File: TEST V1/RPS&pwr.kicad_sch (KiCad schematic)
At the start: 42 parts, among them J10 Conn_01x01_Pin, J12 Conn_01x01_Pin, J7 Conn_01x01_Pin, J8 Conn_01x01_Pin, J9 Conn_01x01_Pin, Q2 PMOS, U11 TVS1800DRV, U12 TPS54202DDC, U13 MCP4725A2T-ECH, U6 LM2596T-5

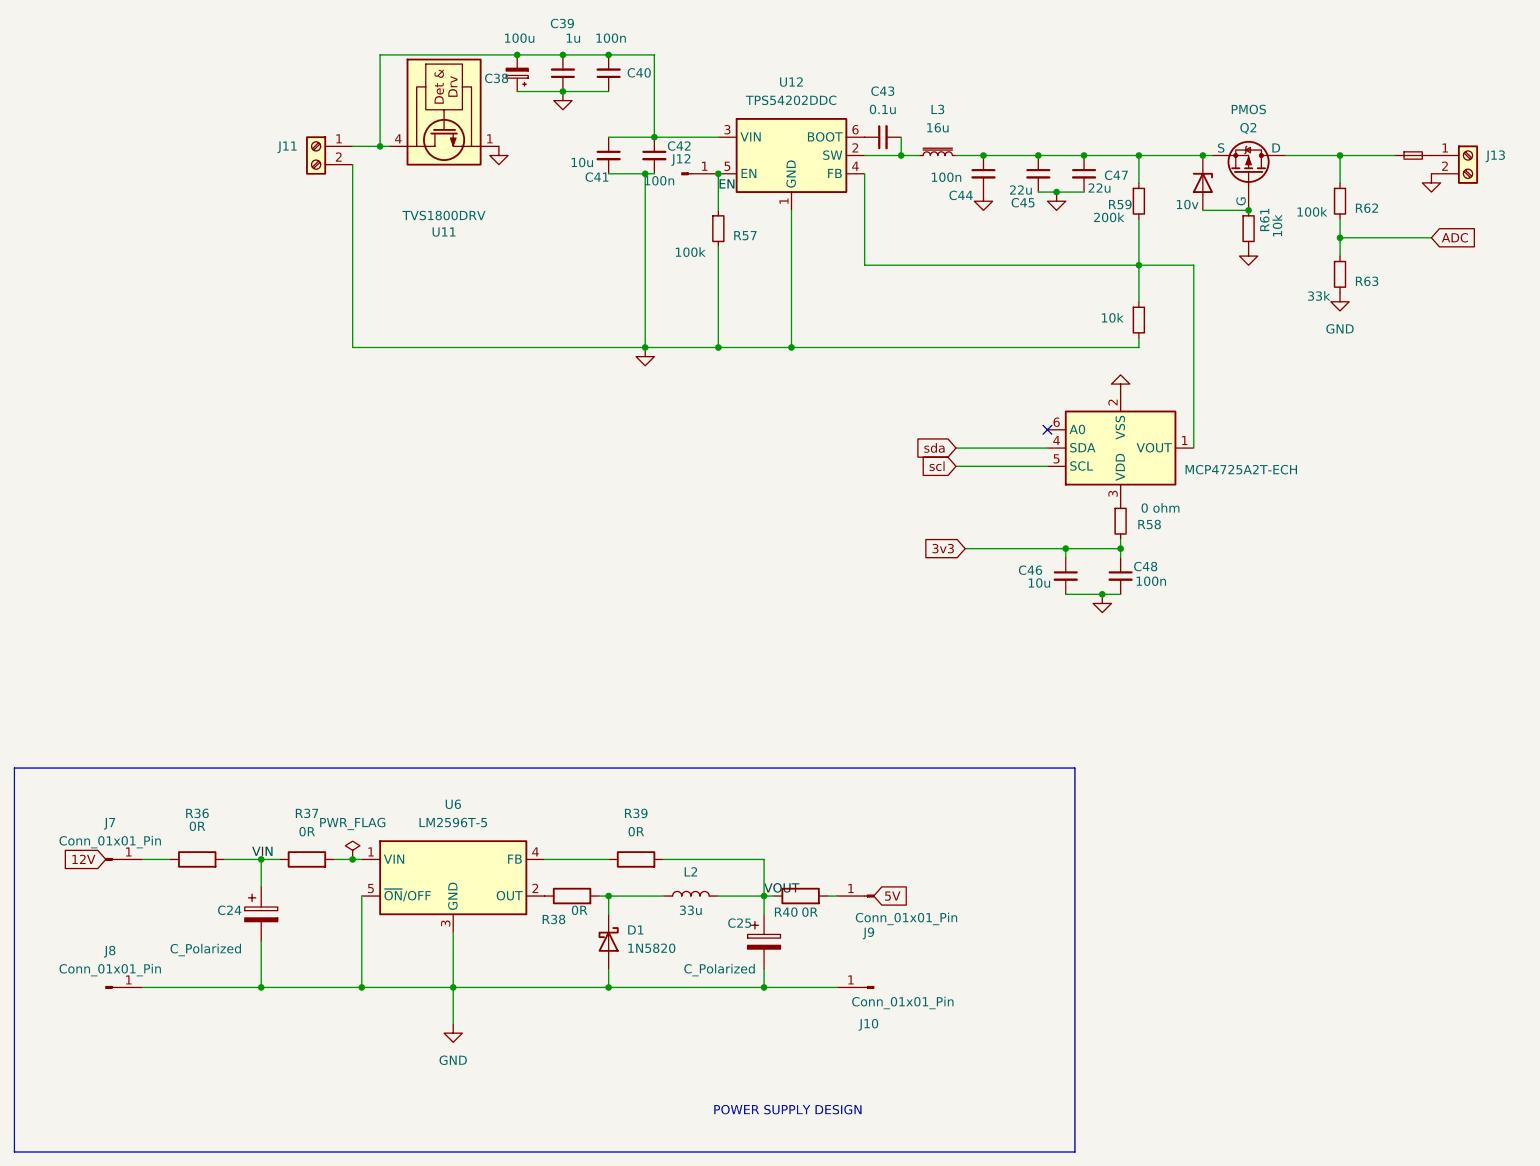
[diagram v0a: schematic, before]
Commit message: updated RPS sch
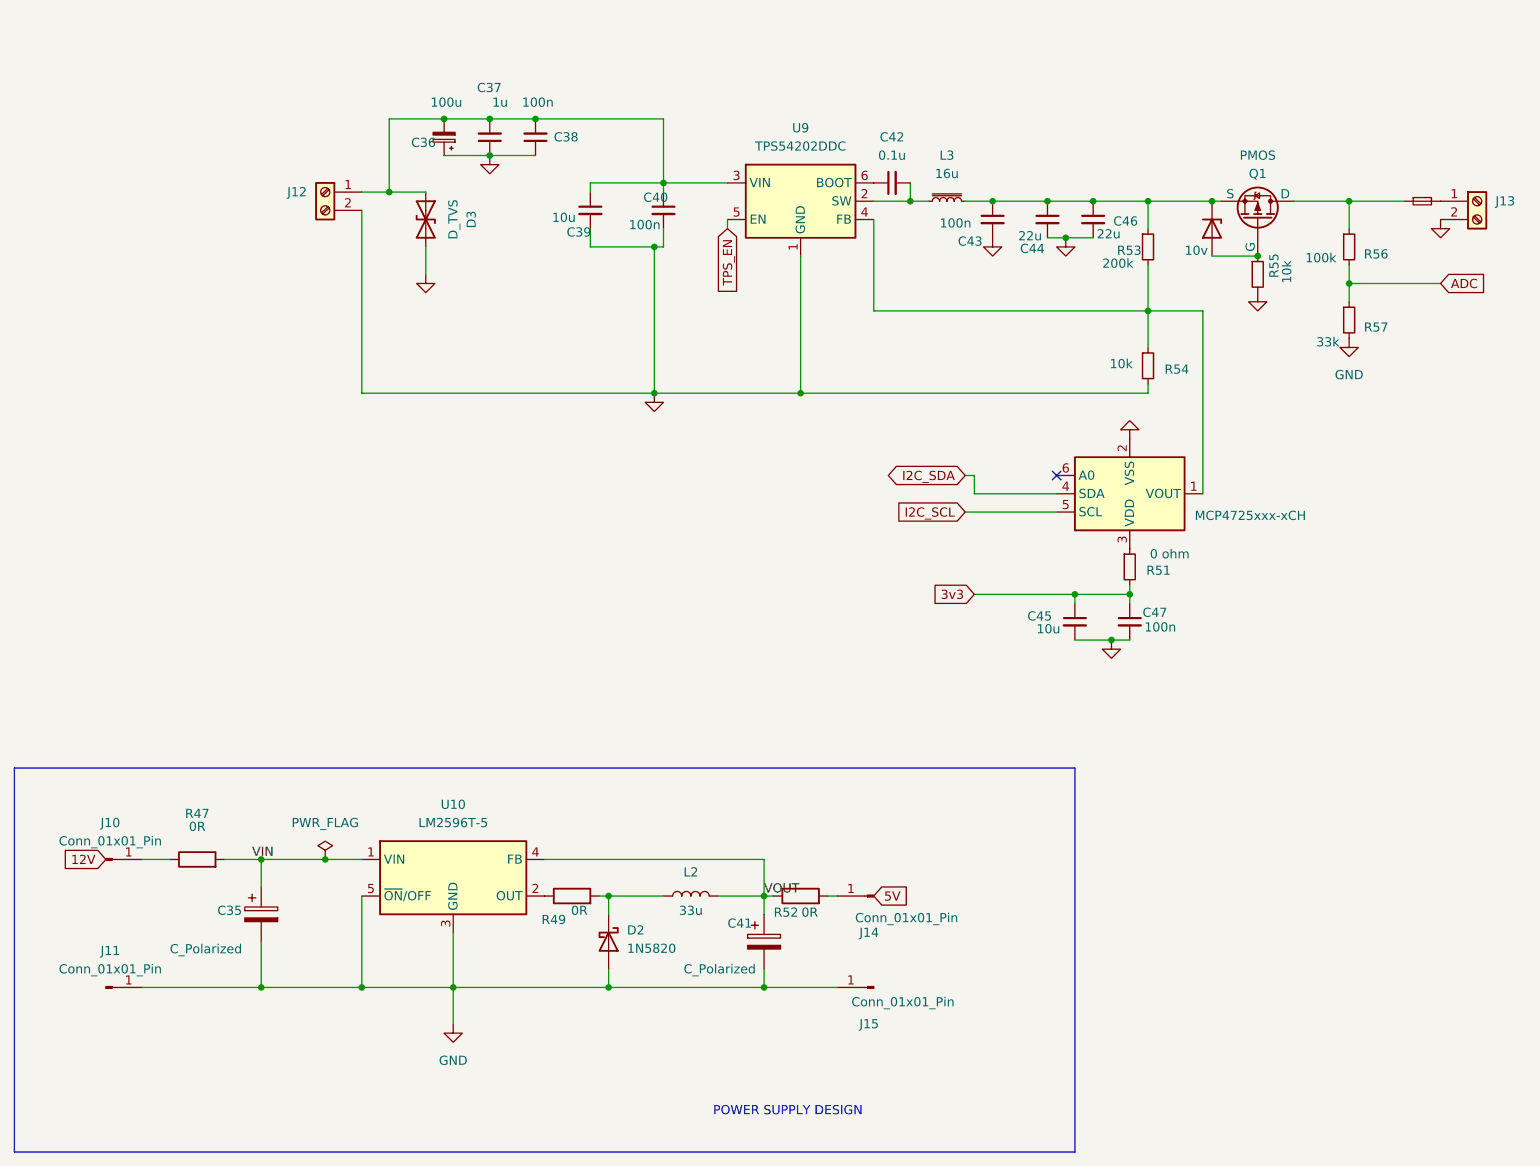
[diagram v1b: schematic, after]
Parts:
- removed C38: 100u, Capacitor_SMD:CP_Elec_6.3x8, symbol Device:C_Polarized_Small
- removed C41: 10u, Capacitor_SMD:C_0603_1608Metric_Pad1.08x0.95mm_HandSolder, symbol Device:C_Small
- removed C48: 100n, Capacitor_SMD:C_0603_1608Metric_Pad1.08x0.95mm_HandSolder, symbol Device:C_Small
- removed D3: 10v, Diode_SMD:D_SOD-123, symbol Device:D_Zener
- removed F2: Fuse_Small, Fuse:Fuse_1206_3216Metric, symbol Device:Fuse_Small
- removed J11: ~, TerminalBlock_Phoenix:TerminalBlock_Phoenix_MKDS-1,5-2-5.08_1x02_P5.08mm_Horizontal, symbol Connector:Screw_Terminal_01x02
- removed J12: Conn_01x01_Pin, Connector_PinHeader_2.54mm:PinHeader_1x01_P2.54mm_Vertical, symbol Connector:Conn_01x01_Pin
- removed Q2: PMOS, Package_TO_SOT_SMD:SOT-223-3_TabPin2, symbol Simulation_SPICE:PMOS
- removed R37, R39: 0R, Resistor_SMD:R_0603_1608Metric_Pad0.98x0.95mm_HandSolder, symbol Device:R
- removed R58: 0 ohm, Resistor_SMD:R_0805_2012Metric_Pad1.20x1.40mm_HandSolder, symbol Device:R_Small
- removed R59: 200k, Resistor_SMD:R_0603_1608Metric_Pad0.98x0.95mm_HandSolder, symbol Device:R_Small
- removed R60, R61: 10k, Resistor_SMD:R_0603_1608Metric_Pad0.98x0.95mm_HandSolder, symbol Device:R_Small
- removed R62: 100k, Resistor_SMD:R_0603_1608Metric_Pad0.98x0.95mm_HandSolder, symbol Device:R_Small
- removed R63: 33k, Resistor_SMD:R_0603_1608Metric_Pad0.98x0.95mm_HandSolder, symbol Device:R_Small
- removed U11: TVS1800DRV, Diode_SMD:D_SMA, symbol Power_Protection:TVS1800DRV
- removed U12: TPS54202DDC, Package_TO_SOT_SMD:SOT-23-6, symbol Regulator_Switching:TPS54202DDC
- removed U13: MCP4725A2T-ECH, Package_TO_SOT_SMD:SOT-23-6, symbol Analog_DAC:MCP4725xxx-xCH
- added C36: 100u, Capacitor_SMD:CP_Elec_6.3x8, symbol Device:C_Polarized_Small
- added C37: 1u, Capacitor_SMD:C_0603_1608Metric_Pad1.08x0.95mm_HandSolder, symbol Device:C_Small
- added C38: 100n, Capacitor_SMD:C_0603_1608Metric_Pad1.08x0.95mm_HandSolder, symbol Device:C_Small
- added D3: D_TVS, Diode_SMD:D_SMA_Handsoldering, symbol Device:D_TVS
- added D4: 10v, Diode_SMD:D_SOD-123, symbol Device:D_Zener
- added F1: Fuse_Small, Fuse:Fuse_1206_3216Metric, symbol Device:Fuse_Small
- added J12: ~, TerminalBlock_Phoenix:TerminalBlock_Phoenix_MKDS-1,5-2-5.08_1x02_P5.08mm_Horizontal, symbol Connector:Screw_Terminal_01x02
- added Q1: PMOS, Package_TO_SOT_SMD:SOT-223-3_TabPin2, symbol Simulation_SPICE:PMOS
- added R51: 0 ohm, Resistor_SMD:R_0805_2012Metric_Pad1.20x1.40mm_HandSolder, symbol Device:R_Small
- added R53: 200k, Resistor_SMD:R_0603_1608Metric_Pad0.98x0.95mm_HandSolder, symbol Device:R_Small
- added R54, R55: 10k, Resistor_SMD:R_0603_1608Metric_Pad0.98x0.95mm_HandSolder, symbol Device:R_Small
- added R56: 100k, Resistor_SMD:R_0603_1608Metric_Pad0.98x0.95mm_HandSolder, symbol Device:R_Small
- added U11: MCP4725xxx-xCH, Package_TO_SOT_SMD:SOT-23-6, symbol Analog_DAC:MCP4725xxx-xCH
- added U9: TPS54202DDC, Package_TO_SOT_SMD:SOT-23-6, symbol Regulator_Switching:TPS54202DDC
- C39: value 1u -> 10u
- C42: value 100n -> 0.1u
- C43: value 0.1u -> 100n
- C44: value 100n -> 22u; footprint Capacitor_SMD:C_0603_1608Metric_Pad1.08x0.95mm_HandSolder -> Capacitor_SMD:C_0805_2012Metric_Pad1.18x1.45mm_HandSolder
- C45: value 22u -> 10u; footprint Capacitor_SMD:C_0805_2012Metric_Pad1.18x1.45mm_HandSolder -> Capacitor_SMD:C_0603_1608Metric_Pad1.08x0.95mm_HandSolder
- C46: value 10u -> 22u; footprint Capacitor_SMD:C_0603_1608Metric_Pad1.08x0.95mm_HandSolder -> Capacitor_SMD:C_0805_2012Metric_Pad1.18x1.45mm_HandSolder
- C47: value 22u -> 100n; footprint Capacitor_SMD:C_0805_2012Metric_Pad1.18x1.45mm_HandSolder -> Capacitor_SMD:C_0603_1608Metric_Pad1.08x0.95mm_HandSolder
- R57: value 100k -> 33k
- renumbered C24 to C35, C25 to C41, D1 to D2, J7 to J10, J8 to J11, J9 to J14, J10 to J15, R36 to R47, R38 to R49, R40 to R52, U6 to U10
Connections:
- net EN is gone; now on net ADC: R57.1
- net 3v3: now also C45.1, C47.1, R51.2; no longer C46.1
- net ADC: now also R56.2
- net GND: now also C39.2, C40.2, C43.2, C36.1, C37.1, C38.1, D3.2 (A2), J12.2 (Pin_2), R54.2, R55.2, U11.2 (VSS), U9.1 (GND); no longer C39.1, C40.1, C42.2
- net VIN: now also U10.1 (VIN)
- net VOUT: now also U10.4 (FB)
- net at C43.1: now also C44.1, C46.1, L3.2, D4.1 (K), Q1.3 (S), R53.1
- net at L3.1: now also C42.2, U9.2 (SW); no longer C43.2
- net at J13.1 (Pin_1): now also F1.2
- new net: C36.2, C37.2, C38.2, C39.1, C40.1, D3.1 (A1), J12.1 (Pin_1), U9.3 (VIN)
- new net: F1.1, Q1.1 (D), R56.1
- new net: D4.2 (A), Q1.2 (G), R55.1
- new net: R53.2, R54.1, U11.1 (VOUT), U9.4 (FB)
- new net: R51.1, U11.3 (VDD)
- new net: C42.1, U9.6 (BOOT)
- new net I2C_SCL: U11.5 (SCL)
- new net I2C_SDA: U11.4 (SDA)
- new net TPS_EN: U9.5 (EN)
